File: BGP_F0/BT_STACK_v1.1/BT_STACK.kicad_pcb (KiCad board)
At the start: 2 copper layers, 24 x 26 mm, 20 parts, among them P1 CONN_01X05, P2 CONN_01X02, P3 CONN_01X04, U1 MC33178

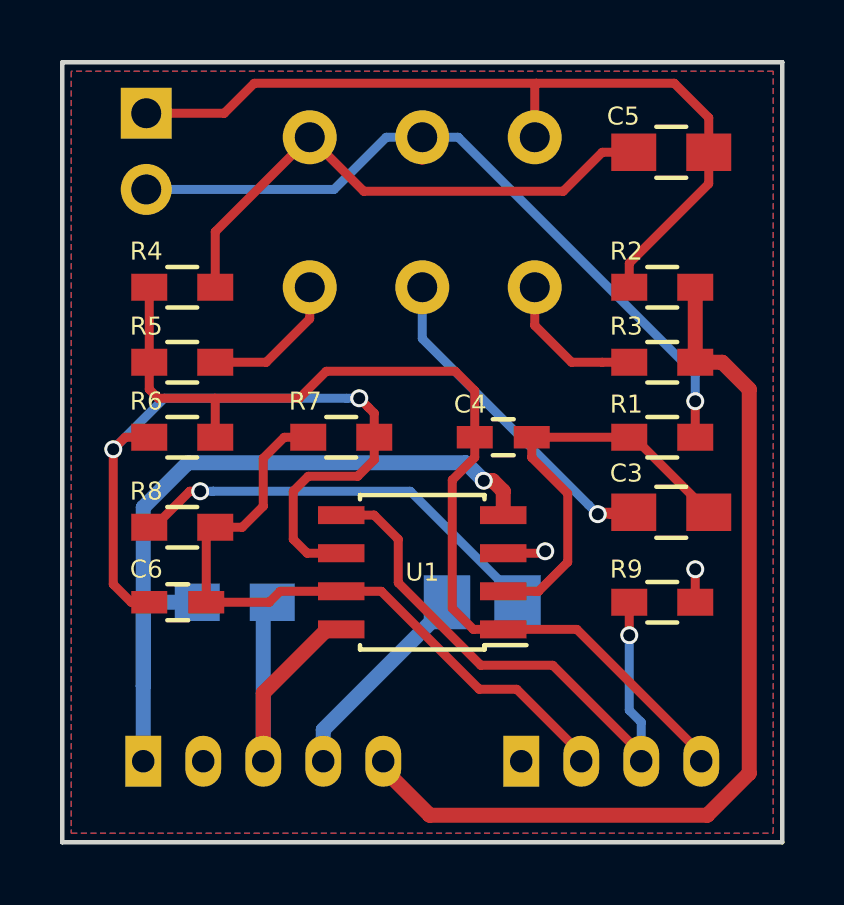
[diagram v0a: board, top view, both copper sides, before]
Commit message: F0 Gerbers
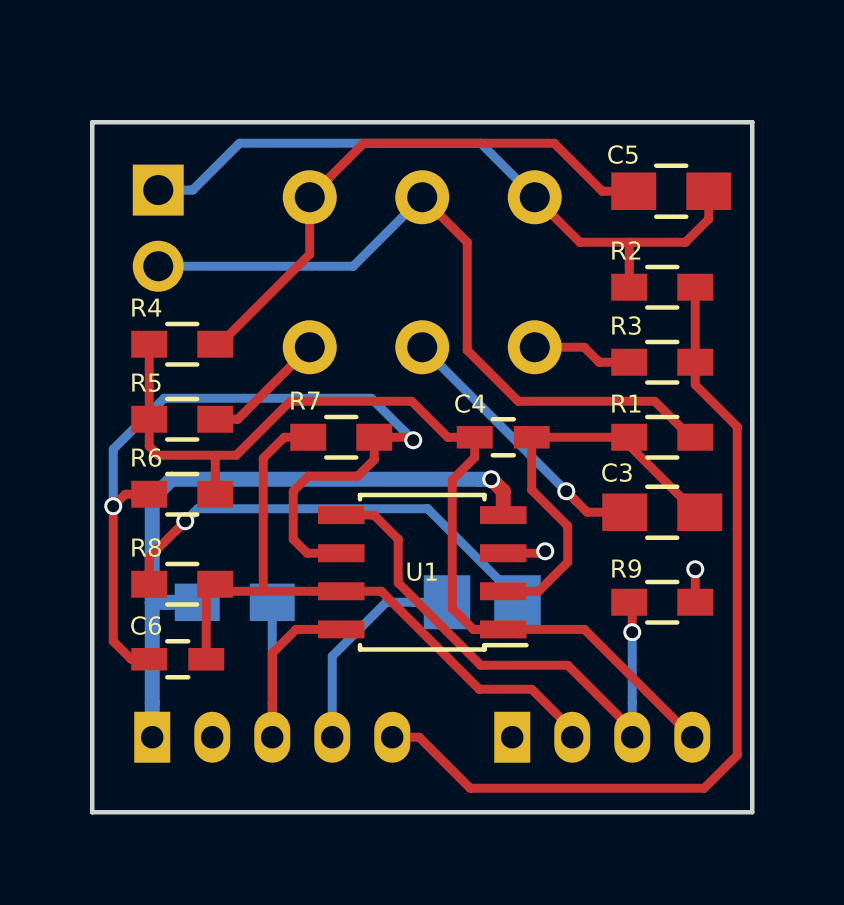
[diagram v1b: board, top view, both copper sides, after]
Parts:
- moved P2 2.59 mm to (143.2, 73.3)
- moved RV1 2.00 mm to (148.2, 73.5)
- moved C6 1.90 mm to (143.8, 88.9)
- moved R4 1.90 mm to (144.0, 78.4)
- moved R5 1.90 mm to (144.0, 80.9)
- moved R6 1.90 mm to (144.0, 83.4)
- moved R8 1.90 mm to (144.0, 86.4)
- moved C5 1.30 mm to (160.3, 73.3)
- moved P1 0.85 mm to (143.0, 91.5)
- moved P3 0.85 mm to (155.0, 91.5)
- moved C3 0.30 mm to (160.0, 84.0)
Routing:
- net /B+: track 28.2 -> 23.1 mm
- net Earth: track 26.9 -> 22.4 mm
- net Net-(C6-Pad2): track 25.2 -> 29.1 mm
- net /TW: track 12.3 -> 9.03 mm
- net /T+: track 6.20 -> 3.36 mm
- net /IN: track 31.1 -> 28.8 mm
- net /MID_R: track 19.9 -> 18.3 mm
- net /BW: track 25.7 -> 24.3 mm, vias 1 -> 0
- net /B-: track 19.6 -> 18.5 mm
- net /MID_I: track 34.4 -> 33.5 mm
- net Net-(C2-Pad1): track 14.4 -> 15.2 mm
- net /V+: track 11.2 -> 10.4 mm
- net /T-: track 4.80 -> 4.14 mm
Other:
- board size 24 x 26 mm -> 22 x 23 mm
